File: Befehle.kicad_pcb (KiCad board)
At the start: 2 copper layers, 100 x 160 mm, 61 parts, among them J1 2PinTerminalBlocktg, J2 2PinTerminalBlocktg, J3 3PinTerminalBlocktg, J4 2PinTerminalBlocktg, J5 2PinTerminalBlocktg, P1 CONN_02X10, P2 CONN_02X10, U1 74LS14, U2 74540, U3 7400, U4 74HCT02, U5 74LS541, U6 74LS373, U7 74LS139, U8 74LS540

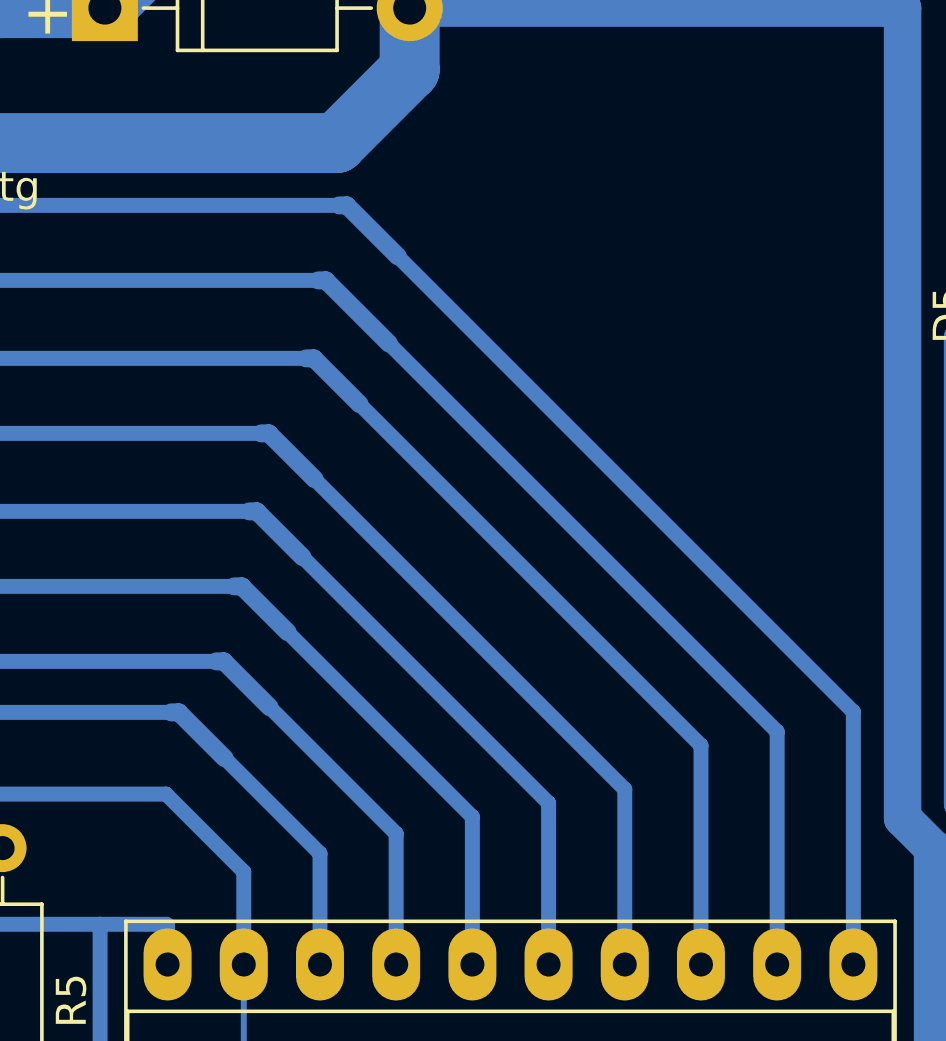
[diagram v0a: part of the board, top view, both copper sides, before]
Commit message: branding
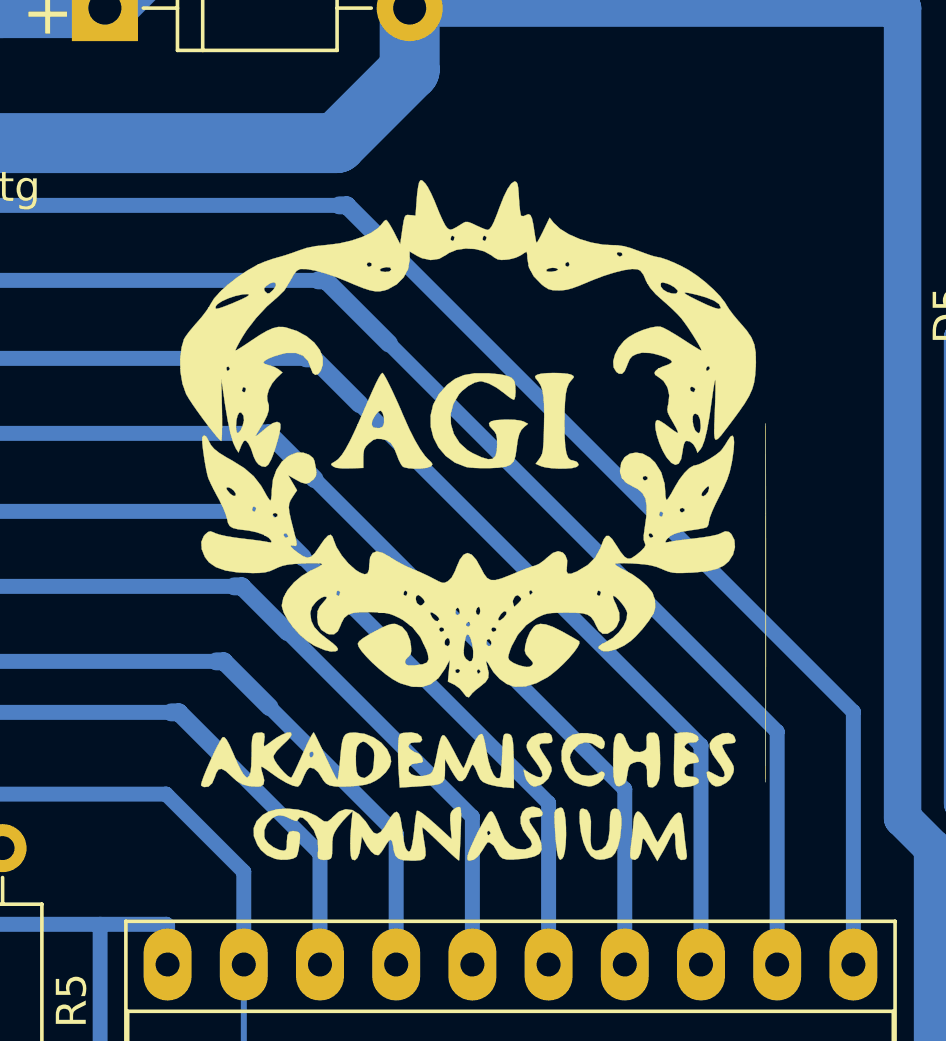
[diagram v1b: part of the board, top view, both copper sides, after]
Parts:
- added G***: LOGO, allBonsaiFootprintsLibs:agi5, F.Cu at (56.0, 45.4)
